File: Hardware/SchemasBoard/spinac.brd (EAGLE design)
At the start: 40.2 x 26.9 mm, 28 parts, among them IC1 LNK304, IC3 MC33269ST-3.3T3, IC4 DS1820, K1 FRS1B, T1 BC846

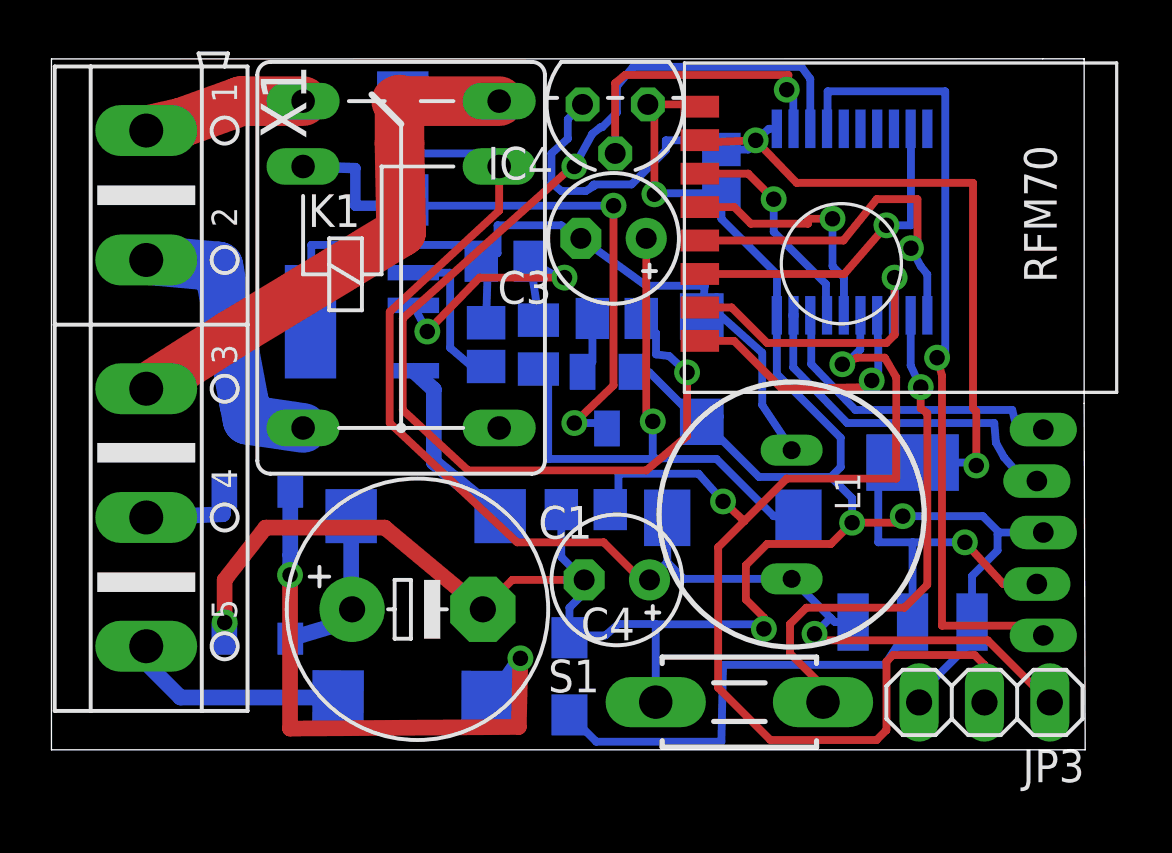
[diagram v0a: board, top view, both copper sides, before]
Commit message: sdfg
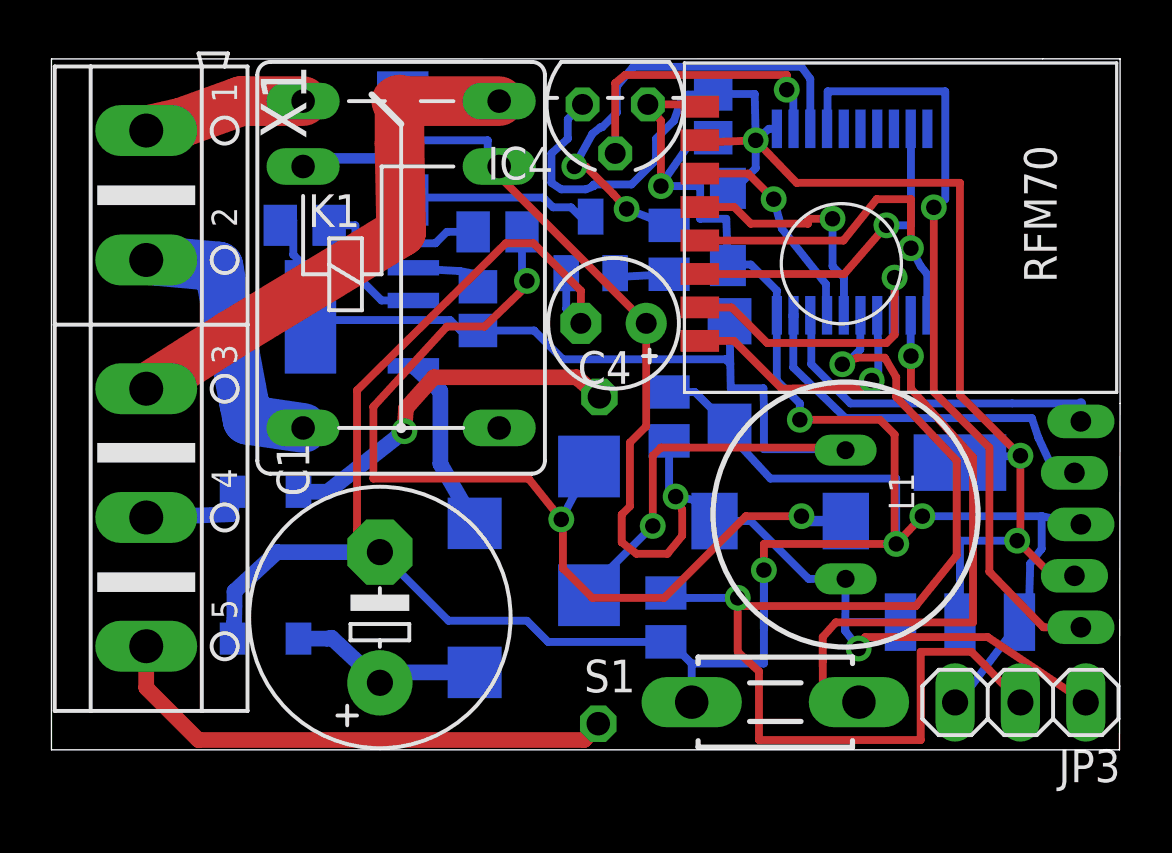
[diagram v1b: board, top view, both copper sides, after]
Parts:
- added R6: 1 K, resistor:M2012
- C3: device resistor:E2,5-5 -> resistor:SMC_C
- R2: device resistor:R2512W -> resistor:0411/12
- moved C6 18.5 mm to (26.3, 20.3), turned to 270 degrees
- moved C3 11.4 mm to (20.9, 8.51), flipped to the bottom, turned to 270 degrees
- moved C4 9.97 mm to (21.8, 16.6)
- moved R2 8.99 mm to (21.3, 7.37), turned to 90.2 degrees
- moved R4 7.93 mm to (9.84, 20.4)
- moved T1 6.07 mm to (21.0, 19.6), turned to 0 degrees
- moved R7 5.22 mm to (23.9, 5.14), turned to 90 degrees
- moved R3 4.66 mm to (17.3, 20.1), turned to 0 degrees
- moved R1 3.70 mm to (16.4, 5.91), turned to 90 degrees
- moved R5 3.35 mm to (24.0, 19.4), turned to 90 degrees
- moved C5 2.18 mm to (25.7, 24.6)
- moved L1 2.10 mm to (30.9, 9.14)
- moved D4 1.85 mm to (28.3, 8.89)
- moved IC3 1.84 mm to (35.3, 8.06)
- moved U$3 1.49 mm to (40.0, 8.76)
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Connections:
- net GND: now also R6.1
- net N$26: now also R6.2
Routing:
- net GND: track 93.1 -> 121.7 mm
- net N$35: track 44.4 -> 18.3 mm
- net N$9: track 23.5 -> 38.5 mm, vias 1 -> 3
- net N$28: track 70.8 -> 56.9 mm
- net N$13: track 33.1 -> 45.3 mm, vias 0 -> 1
- net N$36: track 9.16 -> 20.3 mm
- net N$14: track 24.4 -> 14.1 mm, vias 2 -> 0
- net N$3: track 22.9 -> 14.2 mm, vias 2 -> 1
- net N$10: track 6.05 -> 2.99 mm
- net N$5: track 20.2 -> 22.9 mm
- net N$19: track 12.3 -> 13.7 mm
- net N$18: track 13.9 -> 15.1 mm
- net N$25: track 31.7 -> 30.5 mm
- net N$2: track 6.80 -> 7.71 mm
- net N$11: track 11.2 -> 10.4 mm, vias 2 -> 0
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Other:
- board size 40.2 x 26.9 mm -> 41.5 x 26.9 mm
